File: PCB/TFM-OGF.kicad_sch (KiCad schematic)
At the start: 24 parts, among them J1 Alimentación, J10 5V Output, J11 3.3V Output, J2 CAN_Externo, J3 Jumper CAN, J4 Jumper CAN, J5 Lado izquierdo, J6 Lado derecho, J7 Lado izquierdo, J8 Lado derecho, J9 Led_Pow_Ext, U1 SN65HVD230, U2 SN65HVD230

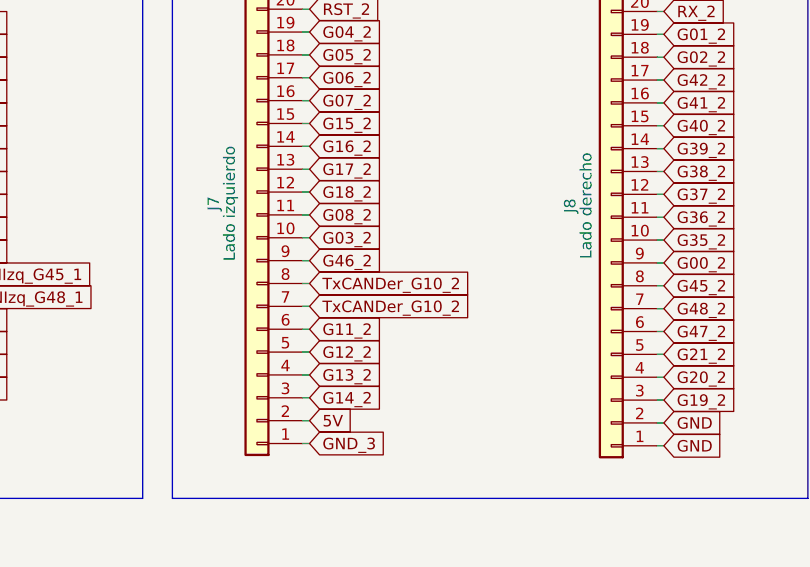
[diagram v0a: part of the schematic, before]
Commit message: Completo placa
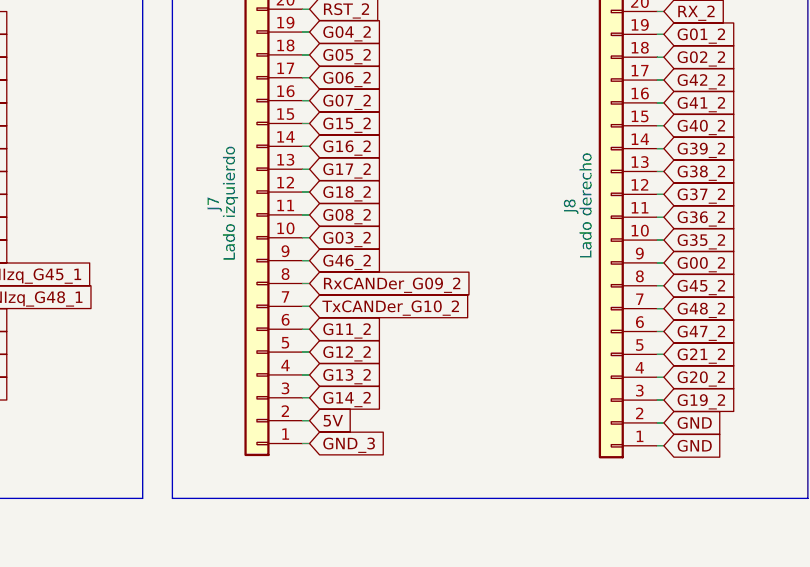
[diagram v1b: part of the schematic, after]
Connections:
- net RxCANDer_G09_2: now also J7.8 (Pin_8)
- net TxCANDer_G10_2: no longer J7.8 (Pin_8)
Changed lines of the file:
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@@
 		)
 	)
-	(global_label "TxCANDer_G10_2"
+	(global_label "RxCANDer_G09_2"
 		(shape input)
 		(at 203.2 103.124 0)
@@
 		)
 		(property "Intersheetrefs" "${INTERSHEET_REFS}"
-			(at 221.8485 103.124 0)
+			(at 222.1509 103.124 0)
 			(effects
 				(font
